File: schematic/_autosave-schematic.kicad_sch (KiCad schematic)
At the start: 45 parts, among them J2 Conn_01x04_Socket, SW1 SW_Push, U1 STM32H743VITx, U2 AMS1117, U3 TB6612FNG_C_8_EL, U4 MP1584, Y1 Crystal_GND23_Small

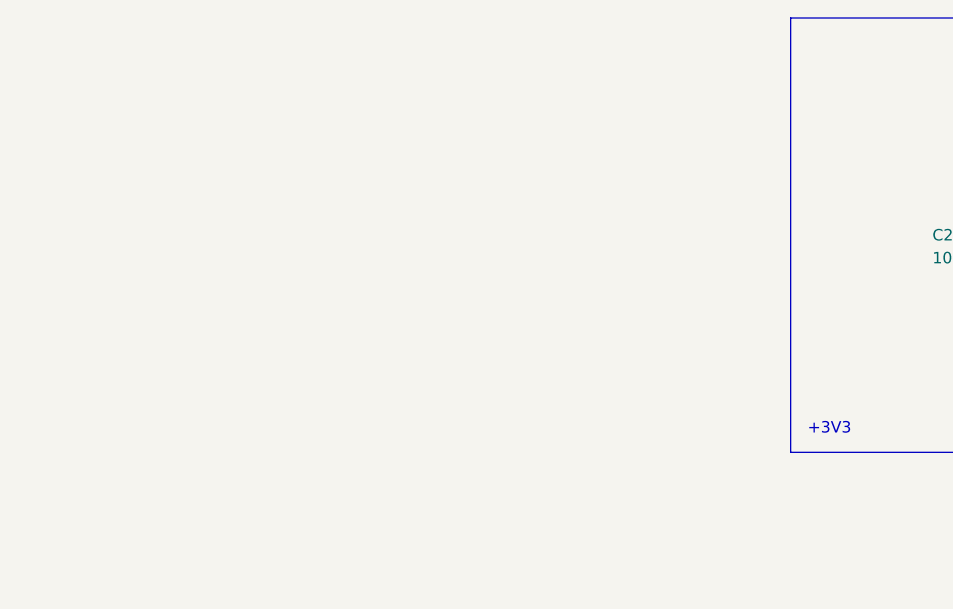
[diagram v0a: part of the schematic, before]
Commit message: no message
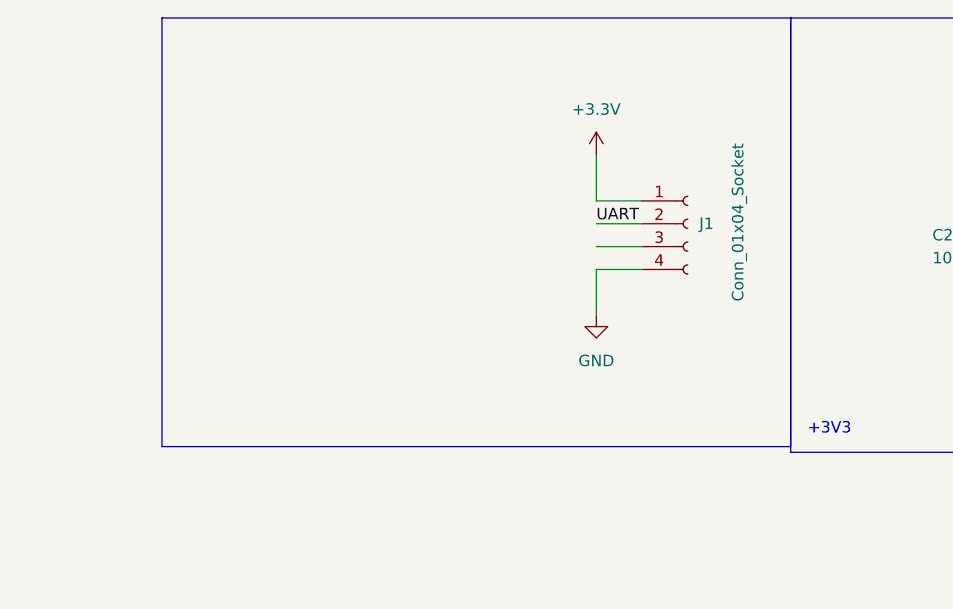
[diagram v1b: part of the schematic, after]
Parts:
- added J1: Conn_01x04_Socket, symbol Connector:Conn_01x04_Socket
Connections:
- net +3.3V: now also J1.1 (Pin_1)
- net GND: now also J1.4 (Pin_4)
- new net UART: J1.2 (Pin_2)
